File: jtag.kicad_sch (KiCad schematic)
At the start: 49 parts, among them J3 USB_C_Receptacle, J4 Conn_01x02_Male, J5 3220-10-0100-00, U2 FT2232HL-REEL, U4 74LVC1G125, U5 74LVC1G125, U6 74LVC1G125, U7 74LVC1G125, U8 74LVC1G125, Y2 12MHz

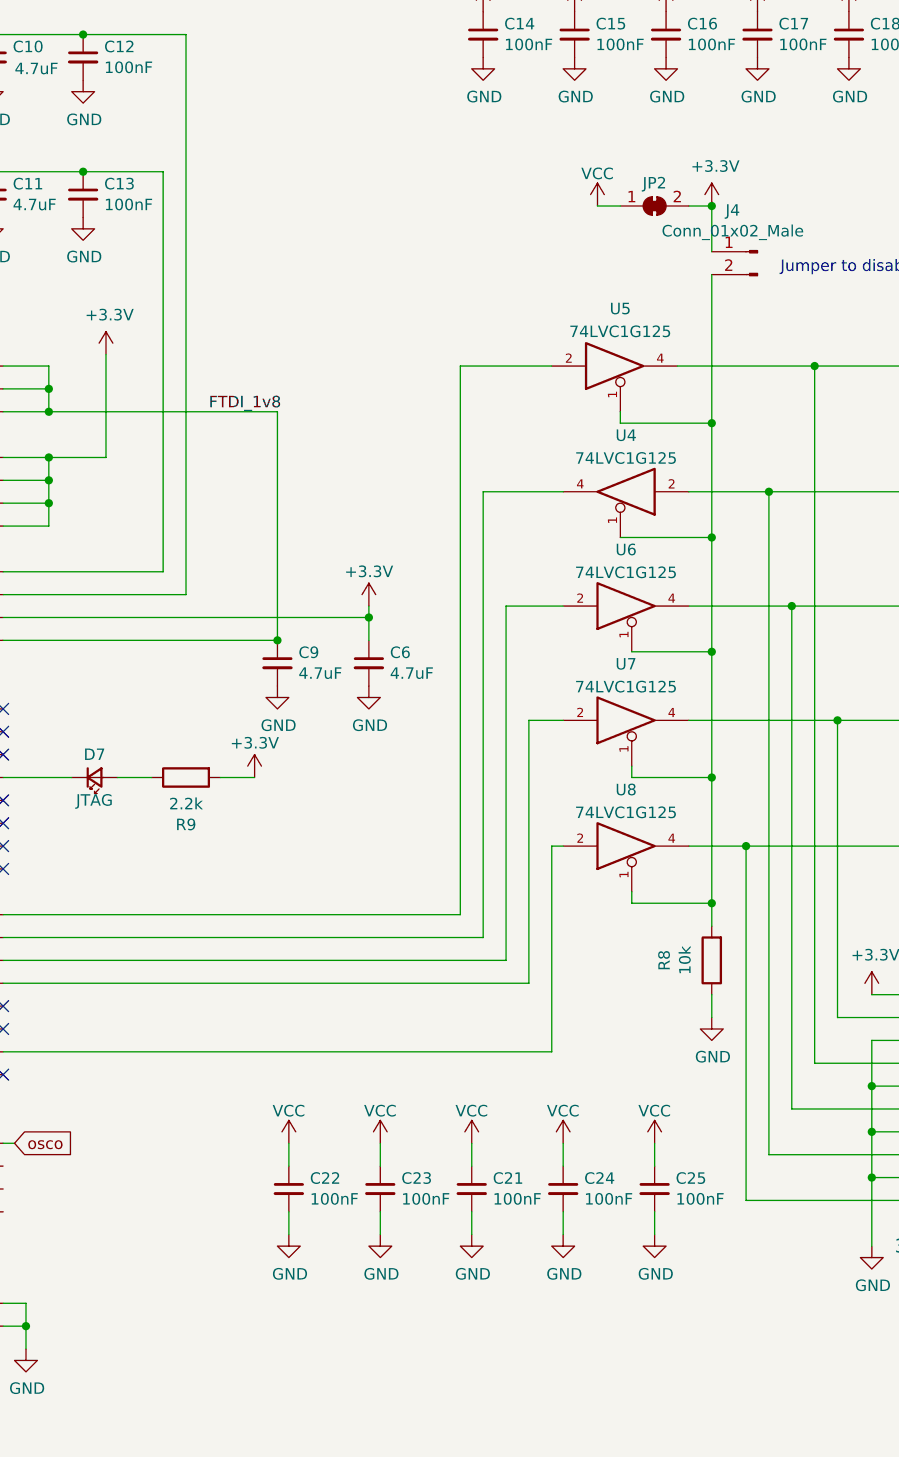
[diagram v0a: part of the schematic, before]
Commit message: Edits to JTAG
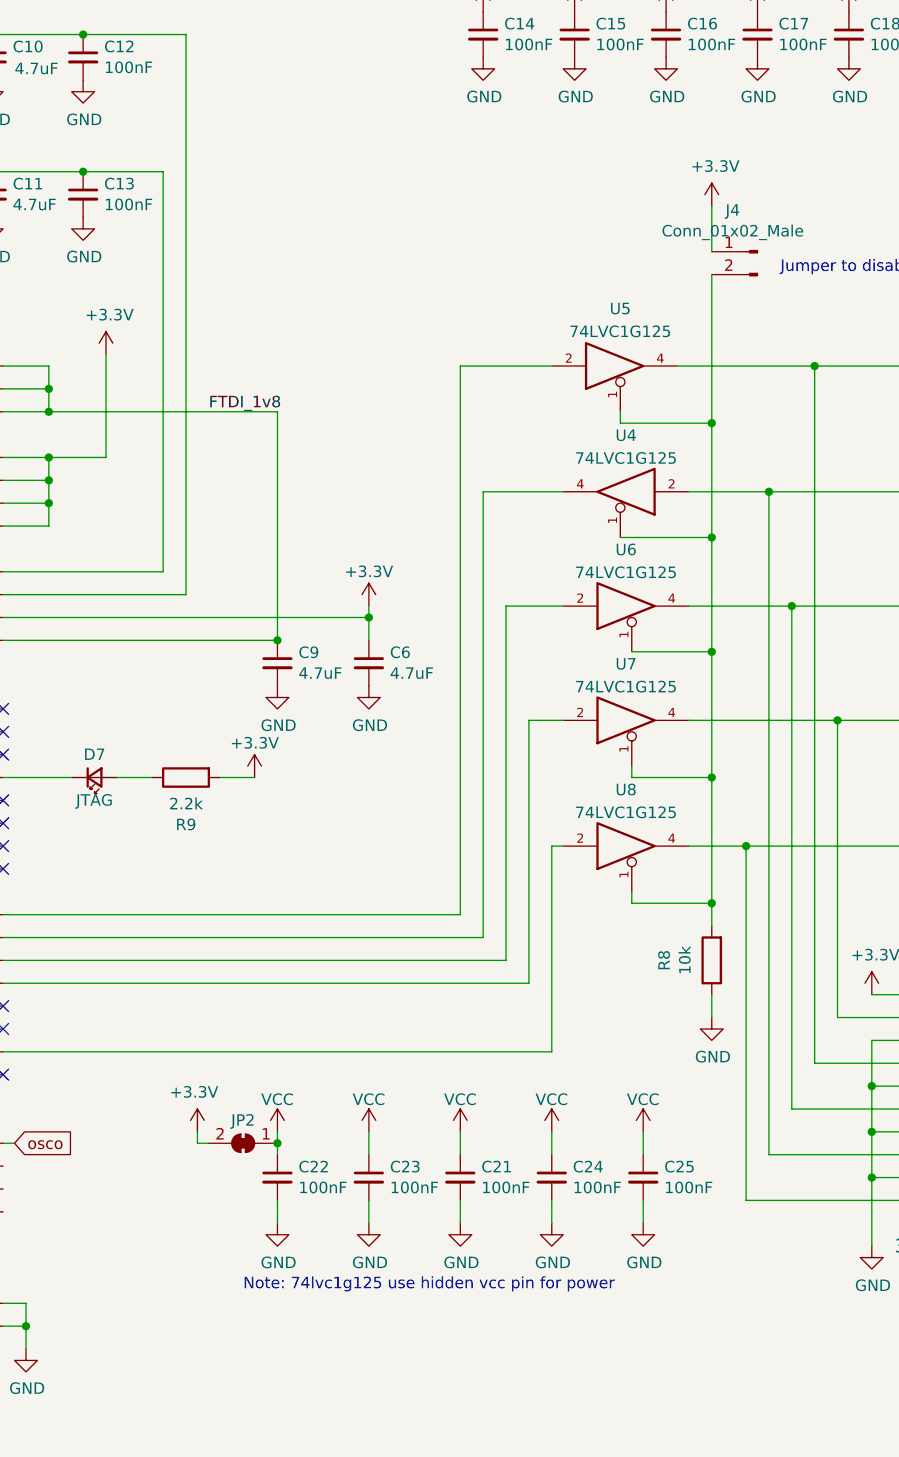
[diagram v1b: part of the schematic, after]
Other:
- note added: "Note: 74lvc1g125 use hidden vcc pin for power"
- moved on the sheet: C21, C22, C23, C24, C25
